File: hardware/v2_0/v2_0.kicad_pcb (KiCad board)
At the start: 4 copper layers, 85 x 68 mm, 107 parts, among them J1 USB_B_Mini, J10 SERV1, J11 SERV2, J12 SPI, J13 UART5, J14 NRFGPIO, J15 USB_B_Mini, J16 DRV1_MTR2, J17 DAC, J18 USB_A, J19 MTR1_CON, J2 CAN, J3 PWR, J4 Power_terminal, J5 DRV1_MTR1, J6 DRV1_MTR2, J7 MTR2_CON, J8 DRV1_MTR1, J9 USART3_UART4, P1 SWD, P2 NRFSWD, Q1 Q_NMOS_GSD, Q2 Q_NMOS_GSD, SW1 MCU_USB_POWER, SW2 NRF_USB_POWER, SW3 BOOT0, U1 TJA1051TK-3, U10 DRV8848, U2 STM32F40X_LQFP64, U3 BMI160, U4 MCP16311/2, U5 DRV8848, U8 BMD-340-A-R, U9 ADP2303ARDZ-5.0, Y1 8M

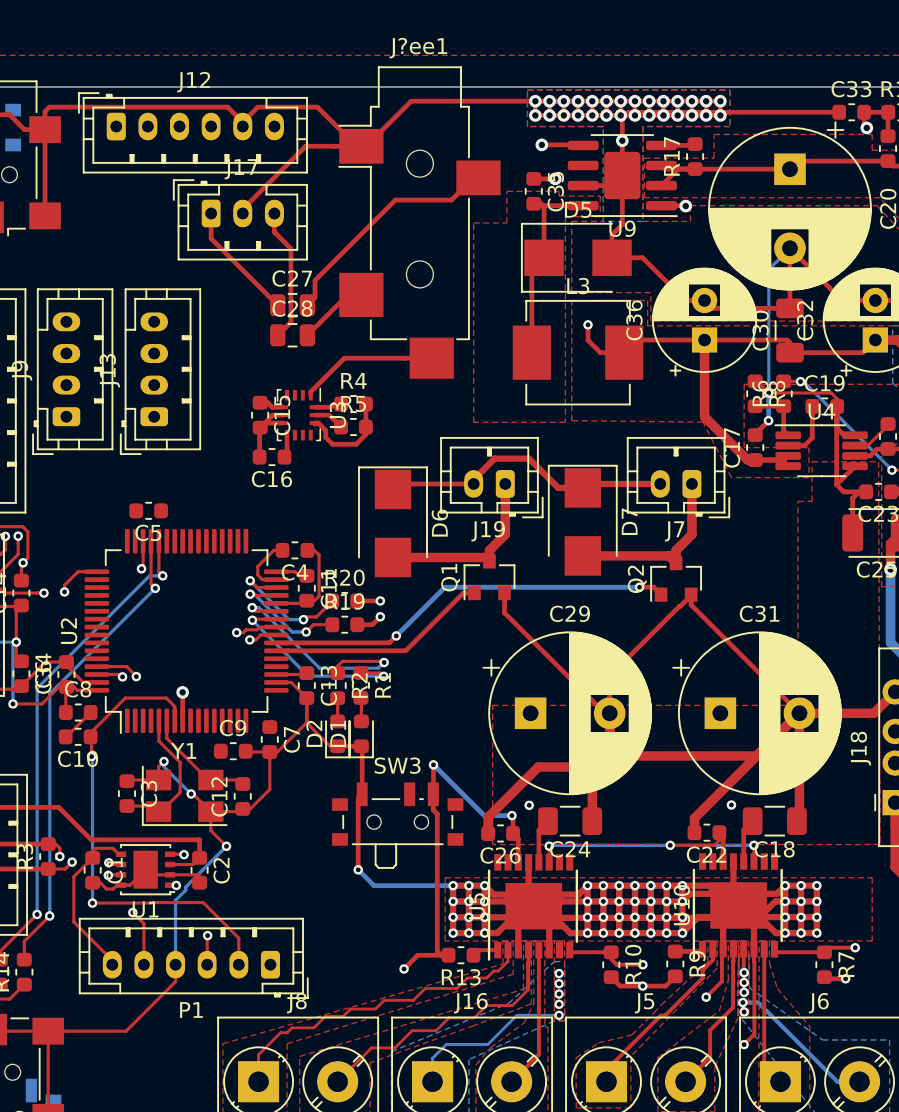
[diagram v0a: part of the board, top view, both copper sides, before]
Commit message: routing some
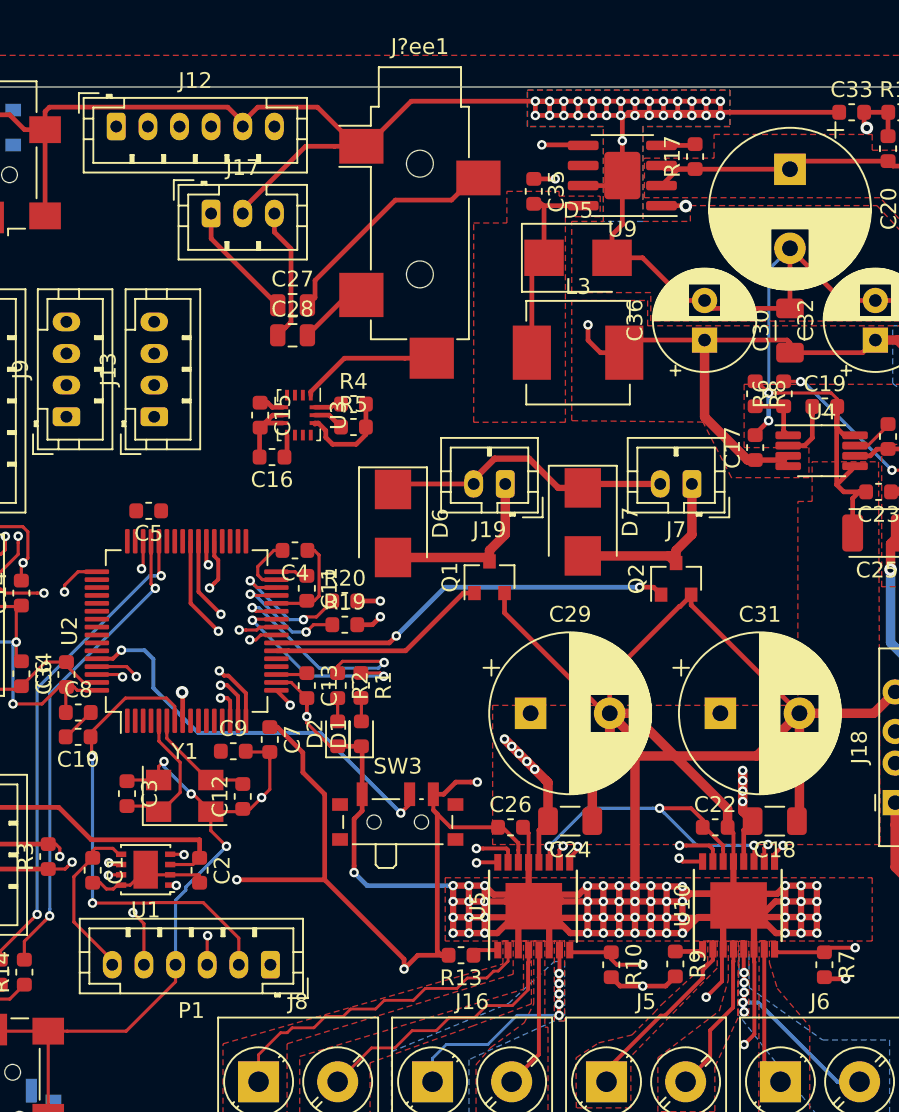
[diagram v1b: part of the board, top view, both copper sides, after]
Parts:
- moved C26 0.74 mm to (204.1, 88.8), turned to 0 degrees
- moved C22 0.62 mm to (217.1, 88.8), turned to 0 degrees
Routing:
- net /DRV1_B1: track 0.00 -> 48.8 mm, vias 0 -> 2
- net /DRV1_A2: track 0.00 -> 39.7 mm, vias 0 -> 2
- net /DRV1_A1: track 0.00 -> 37.0 mm, vias 0 -> 2
- net /DRV2_B1: track 0.00 -> 36.4 mm, vias 0 -> 2
- net /DRV1_B2: track 0.00 -> 36.3 mm, vias 0 -> 2
- net /DRV2_B2: track 0.00 -> 36.0 mm, vias 0 -> 2
- net /DRV2_A2: track 0.00 -> 35.1 mm, vias 0 -> 2
- net /DRV2_A1: track 0.00 -> 34.6 mm, vias 0 -> 2
- net VCC: track 195.8 -> 225.4 mm
- net /base_sheet/BOOT0: track 0.00 -> 26.2 mm, vias 0 -> 2
- net GND: track 698.9 -> 711.4 mm, vias 92 -> 94
- net V_IN: track 157.5 -> 163.0 mm, vias 28 -> 35
- net Net-(J16-Pad1): track 10.6 -> 15.4 mm
- net /DRV1_NFAULT: track 60.6 -> 61.3 mm
- net Net-(J6-Pad2): track 12.8 -> 13.5 mm
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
